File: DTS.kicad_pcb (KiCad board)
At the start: 2 copper layers, 145.5 x 110.5 mm, 0 parts

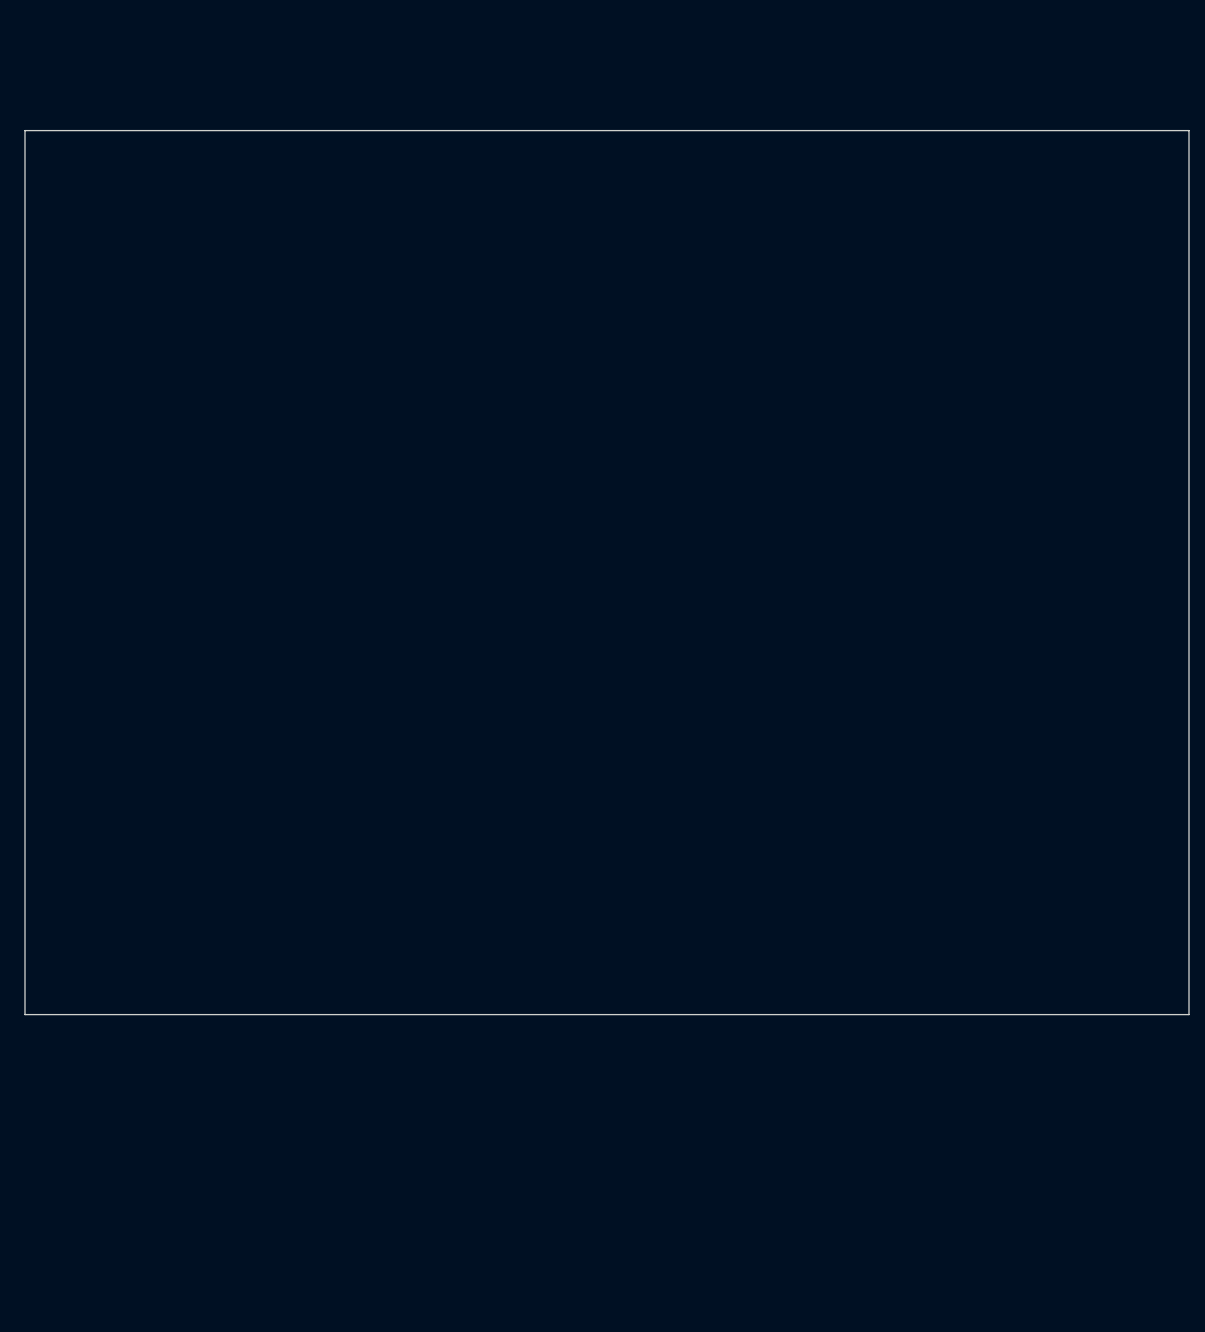
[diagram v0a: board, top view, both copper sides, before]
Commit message: Add files via upload
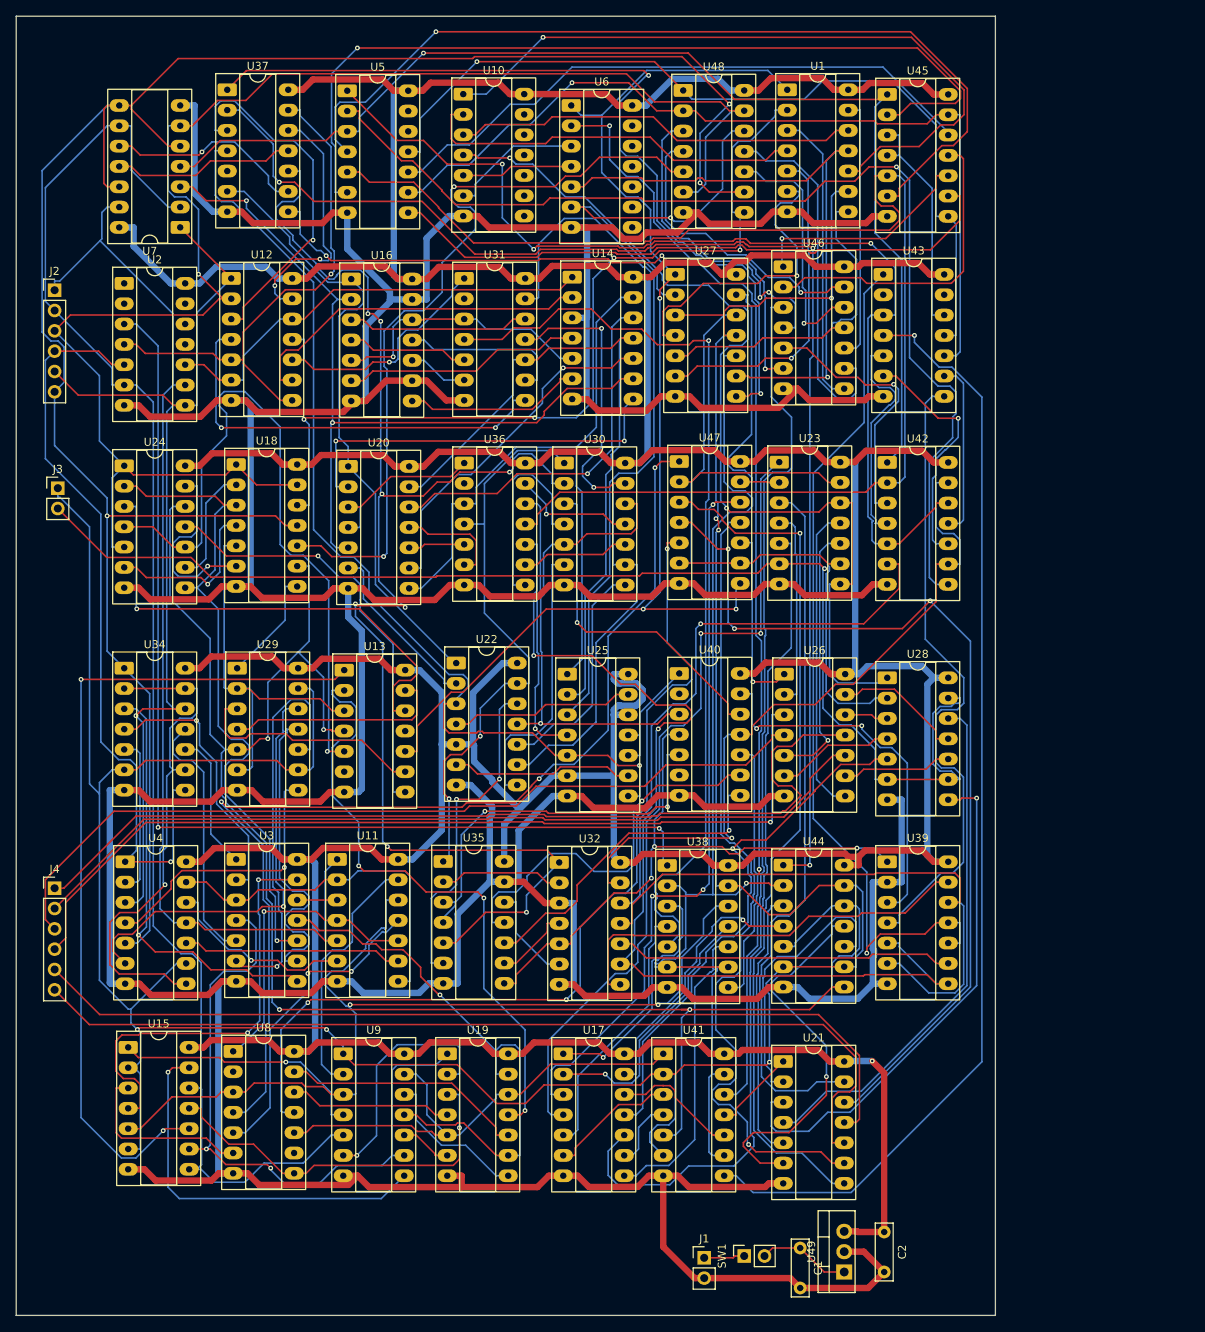
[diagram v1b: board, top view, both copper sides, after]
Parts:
- added C1: 0.22u, Capacitor_THT:C_Rect_L7.0mm_W2.0mm_P5.00mm, F.Cu at (124.4, 173.2)
- added C2: 0.1u, Capacitor_THT:C_Rect_L7.0mm_W2.0mm_P5.00mm, F.Cu at (134.9, 171.2)
- added J1: Conn_01x02_Pin, Connector_PinHeader_2.54mm:PinHeader_1x02_P2.54mm_Vertical, F.Cu at (112.4, 174.4)
- added J2: Conn_01x06_Pin, Connector_PinHeader_2.54mm:PinHeader_1x06_P2.54mm_Vertical, F.Cu at (31.2, 53.5)
- added J3: Conn_01x02_Pin, Connector_PinHeader_2.54mm:PinHeader_1x02_P2.54mm_Vertical, F.Cu at (31.6, 78.2)
- added J4: Conn_01x06_Pin, Connector_PinHeader_2.54mm:PinHeader_1x06_P2.54mm_Vertical, F.Cu at (31.2, 128.2)
- added SW1: SW_DIP_x01, Connector_PinSocket_2.54mm:PinSocket_1x02_P2.54mm_Vertical, F.Cu at (117.4, 174.2)
- added U1: 4081, Package_DIP:CERDIP-14_W7.62mm_SideBrazed_LongPads_Socket, F.Cu at (122.8, 28.4)
- added U10: 4071, Package_DIP:CERDIP-14_W7.62mm_SideBrazed_LongPads_Socket, F.Cu at (82.3, 28.9)
- added U11: 4081, Package_DIP:CERDIP-14_W7.62mm_SideBrazed_LongPads_Socket, F.Cu at (66.5, 124.6)
- added U12: 4081, Package_DIP:CERDIP-14_W7.62mm_SideBrazed_LongPads_Socket, F.Cu at (53.3, 52.0)
- added U13: 4071, Package_DIP:CERDIP-14_W7.62mm_SideBrazed_LongPads_Socket, F.Cu at (67.4, 100.9)
- added U14: 4069, Package_DIP:CERDIP-14_W7.62mm_SideBrazed_LongPads_Socket, F.Cu at (95.9, 51.8)
- added U15: 4081, Package_DIP:CERDIP-14_W7.62mm_SideBrazed_LongPads_Socket, F.Cu at (40.4, 148.1)
- added U16: 4081, Package_DIP:CERDIP-14_W7.62mm_SideBrazed_LongPads_Socket, F.Cu at (68.3, 52.1)
- added U17: 4071, Package_DIP:CERDIP-14_W7.62mm_SideBrazed_LongPads_Socket, F.Cu at (94.8, 148.9)
- added U18: 4069, Package_DIP:CERDIP-14_W7.62mm_SideBrazed_LongPads_Socket, F.Cu at (53.9, 75.2)
- added U19: 4081, Package_DIP:CERDIP-14_W7.62mm_SideBrazed_LongPads_Socket, F.Cu at (80.3, 148.9)
- added U2: 4081, Package_DIP:CERDIP-14_W7.62mm_SideBrazed_LongPads_Socket, F.Cu at (39.9, 52.6)
- added U20: 4081, Package_DIP:CERDIP-14_W7.62mm_SideBrazed_LongPads_Socket, F.Cu at (67.9, 75.5)
- added U21: 4071, Package_DIP:CERDIP-14_W7.62mm_SideBrazed_LongPads_Socket, F.Cu at (122.3, 149.9)
- added U22: 4069, Package_DIP:CERDIP-14_W7.62mm_SideBrazed_LongPads_Socket, F.Cu at (81.4, 100.1)
- added U23: 4081, Package_DIP:CERDIP-14_W7.62mm_SideBrazed_LongPads_Socket, F.Cu at (121.8, 74.9)
- added U24: 4081, Package_DIP:CERDIP-14_W7.62mm_SideBrazed_LongPads_Socket, F.Cu at (39.9, 75.4)
- added U25: 4081, Package_DIP:CERDIP-14_W7.62mm_SideBrazed_LongPads_Socket, F.Cu at (95.3, 101.4)
- added U26: 4071, Package_DIP:CERDIP-14_W7.62mm_SideBrazed_LongPads_Socket, F.Cu at (122.4, 101.4)
- added U27: 4069, Package_DIP:CERDIP-14_W7.62mm_SideBrazed_LongPads_Socket, F.Cu at (108.8, 51.5)
- added U28: 4081, Package_DIP:CERDIP-14_W7.62mm_SideBrazed_LongPads_Socket, F.Cu at (135.3, 101.9)
- added U29: 4081, Package_DIP:CERDIP-14_W7.62mm_SideBrazed_LongPads_Socket, F.Cu at (54.0, 100.7)
- added U3: 4071, Package_DIP:CERDIP-14_W7.62mm_SideBrazed_LongPads_Socket, F.Cu at (53.9, 124.6)
- added U30: 4081, Package_DIP:CERDIP-14_W7.62mm_SideBrazed_LongPads_Socket, F.Cu at (94.9, 75.1)
- added U31: 4071, Package_DIP:CERDIP-14_W7.62mm_SideBrazed_LongPads_Socket, F.Cu at (82.4, 52.0)
- added U32: 4069, Package_DIP:CERDIP-14_W7.62mm_SideBrazed_LongPads_Socket, F.Cu at (94.3, 125.0)
- added U34: 4081, Package_DIP:CERDIP-14_W7.62mm_SideBrazed_LongPads_Socket, F.Cu at (39.9, 100.7)
- added U35: 4081, Package_DIP:CERDIP-14_W7.62mm_SideBrazed_LongPads_Socket, F.Cu at (79.8, 124.9)
- added U36: 4071, Package_DIP:CERDIP-14_W7.62mm_SideBrazed_LongPads_Socket, F.Cu at (82.4, 75.1)
- added U37: 4069, Package_DIP:CERDIP-14_W7.62mm_SideBrazed_LongPads_Socket, F.Cu at (52.8, 28.4)
- added U38: 4081, Package_DIP:CERDIP-14_W7.62mm_SideBrazed_LongPads_Socket, F.Cu at (107.8, 125.4)
- added U39: 4081, Package_DIP:CERDIP-14_W7.62mm_SideBrazed_LongPads_Socket, F.Cu at (135.3, 124.9)
- added U4: 4069, Package_DIP:CERDIP-14_W7.62mm_SideBrazed_LongPads_Socket, F.Cu at (40.0, 124.9)
- added U40: 4071, Package_DIP:CERDIP-14_W7.62mm_SideBrazed_LongPads_Socket, F.Cu at (109.3, 101.4)
- added U41: 4081, Package_DIP:CERDIP-14_W7.62mm_SideBrazed_LongPads_Socket, F.Cu at (107.3, 148.9)
- added U42: 4081, Package_DIP:CERDIP-14_W7.62mm_SideBrazed_LongPads_Socket, F.Cu at (135.3, 75.0)
- added U43: 4071, Package_DIP:CERDIP-14_W7.62mm_SideBrazed_LongPads_Socket, F.Cu at (134.8, 51.5)
- added U44: 4081, Package_DIP:CERDIP-14_W7.62mm_SideBrazed_LongPads_Socket, F.Cu at (122.3, 125.3)
- added U45: 4081, Package_DIP:CERDIP-14_W7.62mm_SideBrazed_LongPads_Socket, F.Cu at (135.3, 29.0)
- added U46: 4071, Package_DIP:CERDIP-14_W7.62mm_SideBrazed_LongPads_Socket, F.Cu at (122.3, 50.5)
- added U47: 4081, Package_DIP:CERDIP-14_W7.62mm_SideBrazed_LongPads_Socket, F.Cu at (109.3, 74.9)
- added U48: 4081, Package_DIP:CERDIP-14_W7.62mm_SideBrazed_LongPads_Socket, F.Cu at (109.8, 28.5)
- added U49: LM7805_TO220, Package_TO_SOT_THT:TO-220-3_Vertical, F.Cu at (129.9, 176.2)
- added U5: 4069, Package_DIP:CERDIP-14_W7.62mm_SideBrazed_LongPads_Socket, F.Cu at (67.8, 28.5)
- added U6: 4081, Package_DIP:CERDIP-14_W7.62mm_SideBrazed_LongPads_Socket, F.Cu at (95.8, 30.4)
- added U7: 4081, Package_DIP:CERDIP-14_W7.62mm_SideBrazed_LongPads_Socket, F.Cu at (46.9, 45.6)
- added U8: 4071, Package_DIP:CERDIP-14_W7.62mm_SideBrazed_LongPads_Socket, F.Cu at (53.5, 148.6)
- added U9: 4069, Package_DIP:CERDIP-14_W7.62mm_SideBrazed_LongPads_Socket, F.Cu at (67.3, 148.9)
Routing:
- net GND: track 0.00 -> 857.9 mm
- net VCC: track 0.00 -> 812.4 mm, vias 0 -> 1
- net ctrl_out0: track 0.00 -> 403.9 mm, vias 0 -> 6
- net y3: track 0.00 -> 263.7 mm, vias 0 -> 3
- net xor3: track 0.00 -> 231.8 mm, vias 0 -> 4
- net /Multiplier/(A1B2)': track 0.00 -> 212.7 mm, vias 0 -> 3
- net ctrl_out1: track 0.00 -> 205.6 mm, vias 0 -> 1
- net x3: track 0.00 -> 196.3 mm, vias 0 -> 1
- net x2: track 0.00 -> 184.0 mm
- net /Multiplier/(A0B2)': track 0.00 -> 178.1 mm, vias 0 -> 8
- net /Multiplier/cout3: track 0.00 -> 173.3 mm
- net /Multiplexer_6b1/i0_5: track 0.00 -> 164.7 mm, vias 0 -> 3
- net s3: track 0.00 -> 152.4 mm, vias 0 -> 3
- net /Multiplier/A2B2: track 0.00 -> 145.8 mm, vias 0 -> 1
- net x1: track 0.00 -> 140.5 mm
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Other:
- board size 145.5 x 110.5 mm -> 122.4 x 162.4 mm
